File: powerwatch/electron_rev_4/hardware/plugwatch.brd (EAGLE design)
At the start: 52.8 x 90.9 mm, 128 parts, among them J1 CON_MICRO_SDDM3AT-SF-PEJM5, U1 BGA725L6-ALT, U10 SIP32510, U12 SIP32510, U13 AB1815-T3, U16 MAX6746, U2 SAFFB1G56KB0F0A, U3 IRM-03-5V, U4 MAX-M8, U5 OPA369, U6 LIS2DW12, U8 OPA369, U9 SIP32510, X1 ABS07-32.768KHZ-7-T

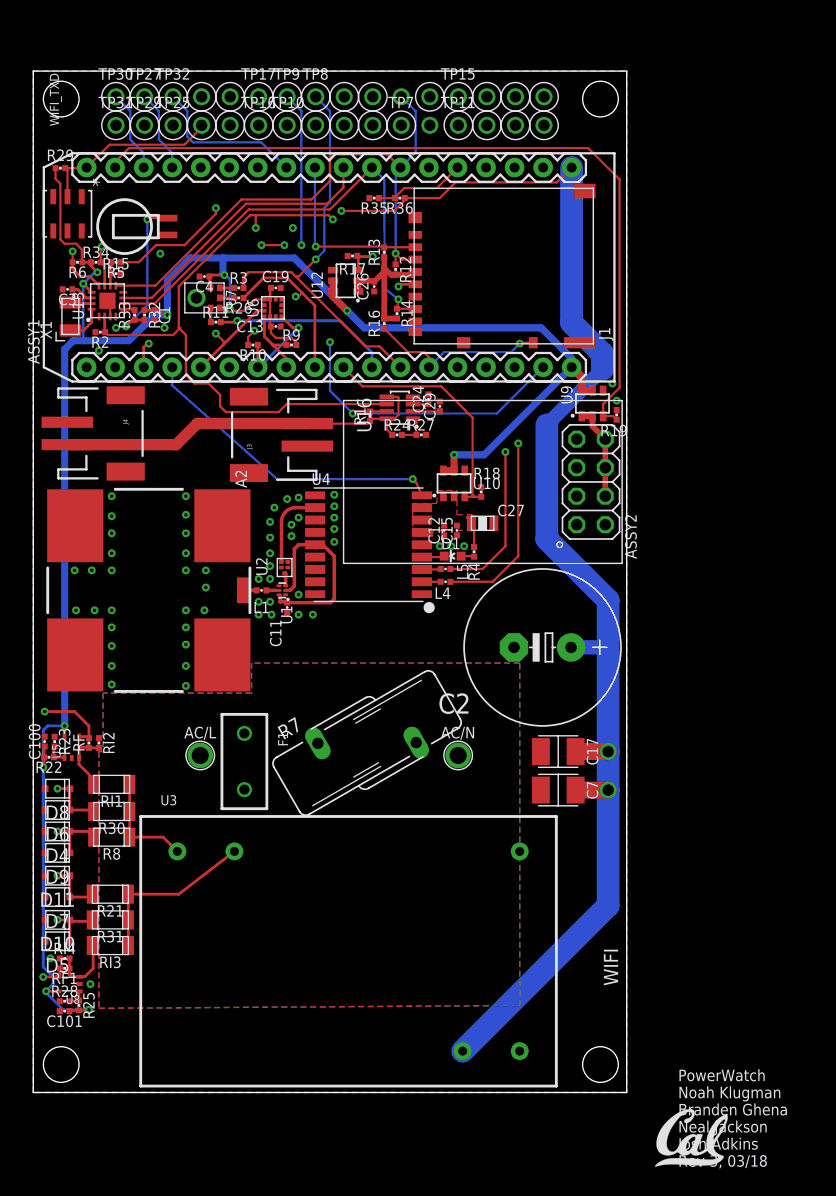
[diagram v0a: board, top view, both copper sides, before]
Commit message: fixed based on case, rerouted, some of the silk
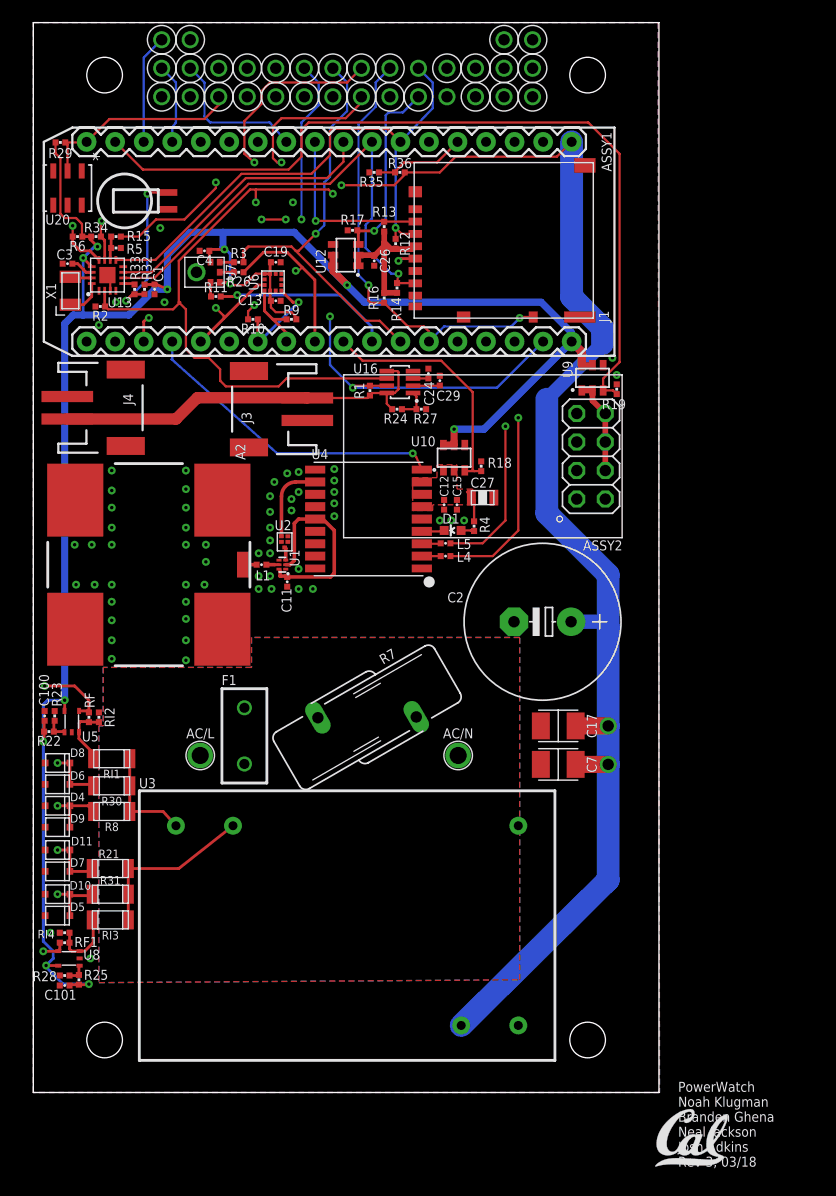
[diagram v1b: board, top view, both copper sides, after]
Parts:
- removed SERIAL: DS2401P+, DS2401P+:21-0382
- added U20: DS2401P+, DS2401P+:21-0382
- moved TP31 10.1 mm to (14.0, 93.7)
- moved TP26 7.69 mm to (44.5, 93.7)
- moved TP30 6.51 mm to (11.4, 93.7)
- moved TP18 6.20 mm to (41.9, 93.7)
- moved TP1 2.96 mm to (44.5, 91.2)
- moved TP11 2.96 mm to (39.4, 88.6)
- moved TP12 2.96 mm to (16.5, 91.2)
- moved TP13 2.96 mm to (19.1, 91.2)
- moved TP14 2.96 mm to (19.1, 88.6)
- moved TP15 2.96 mm to (39.4, 91.2)
- moved TP16 2.96 mm to (21.6, 88.6)
- moved TP17 2.96 mm to (21.6, 91.2)
- moved TP19 2.96 mm to (29.2, 88.6)
- moved TP2 2.96 mm to (44.5, 88.6)
- moved TP20 2.96 mm to (29.2, 91.2)
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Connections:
- net GND: now also U20.1; no longer SERIAL.1
- net SERIAL_NUM: now also U20.2; no longer SERIAL.2
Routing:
- net SENSORS_SCL: track 6.56 -> 42.0 mm, vias 0 -> 1
- net SENSORS_SDA: track 9.03 -> 35.2 mm, vias 1 -> 2
- net !SD_DETECT: track 16.1 -> 39.8 mm, vias 1 -> 2
- net SD_ENABLE: track 28.8 -> 43.3 mm
- net AC/L-SENSE: track 72.6 -> 81.2 mm
- net VCC: track 220.3 -> 225.3 mm
- net WIFI_PWR_EN: track 82.3 -> 87.3 mm
- net !EXTERNAL_RST: track 53.4 -> 56.9 mm
- net SD_MISO: track 51.8 -> 54.4 mm
- net AC/N-SENSE: track 90.6 -> 93.1 mm
- net AC/N-FUSED: track 39.7 -> 41.7 mm
- net WDI: track 75.2 -> 77.2 mm
- net !SD_CS: track 23.2 -> 25.2 mm
- net SERIAL_NUM: track 16.5 -> 18.4 mm
- net WIFI_TXD: track 85.8 -> 87.6 mm
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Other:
- board size 52.8 x 90.9 mm -> 55.7 x 95.2 mm
- board text removed: "WIFI"
- board text removed: "WIFI_TXD"
